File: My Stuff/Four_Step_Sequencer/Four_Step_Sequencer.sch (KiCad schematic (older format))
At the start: 46 parts, among them J1 CK_In, J10 1w, J11 2w, J12 3w, J13 4w, J2 CV_Out, J3 +12V_Conn, J4 GND_Conn, J5 -12V_Conn, J6 1a, J7 2a, J8 3a, J9 4a, U1 TL074, U2 4017

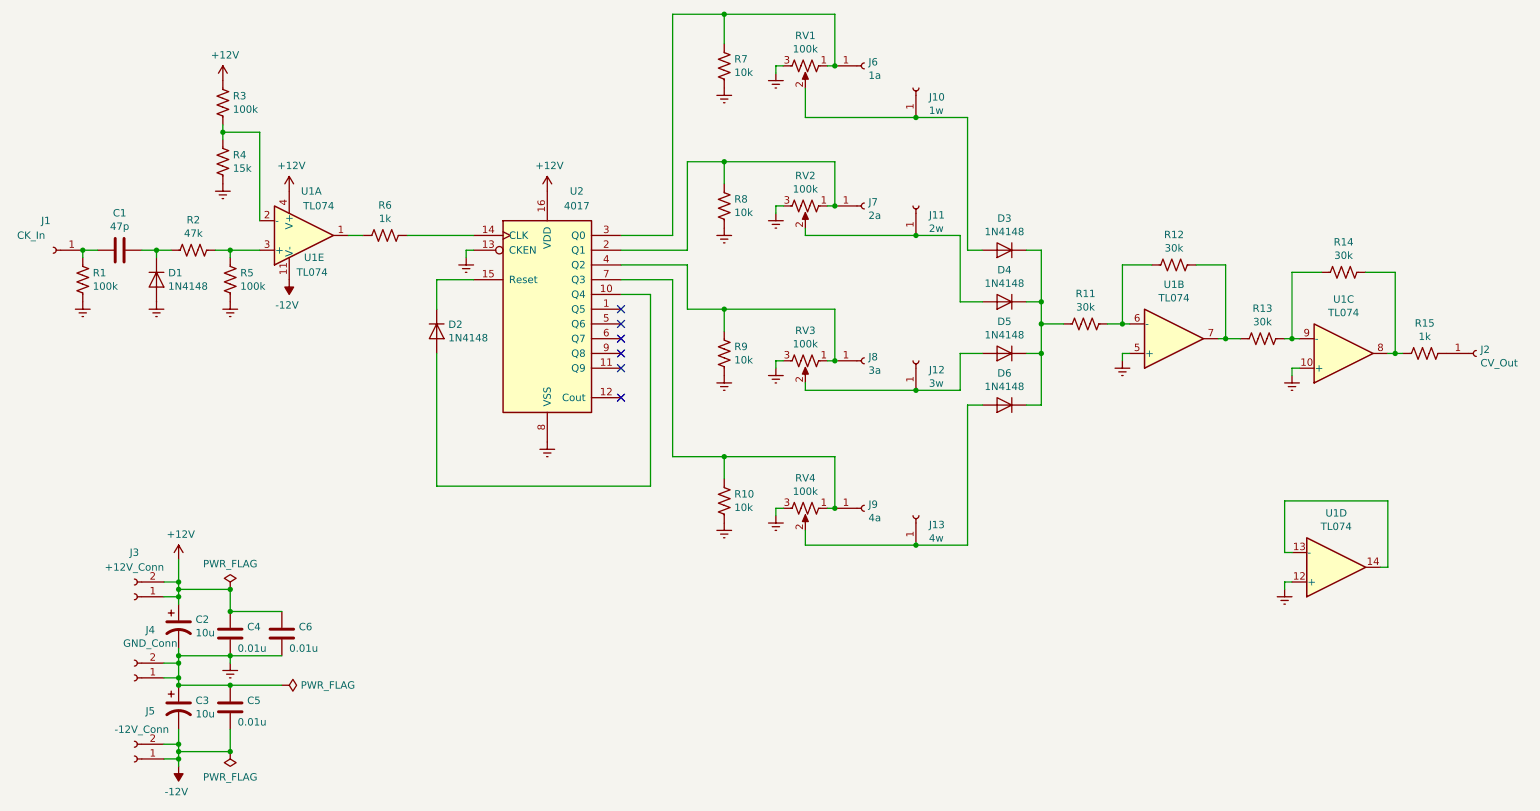
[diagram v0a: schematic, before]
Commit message: uwu
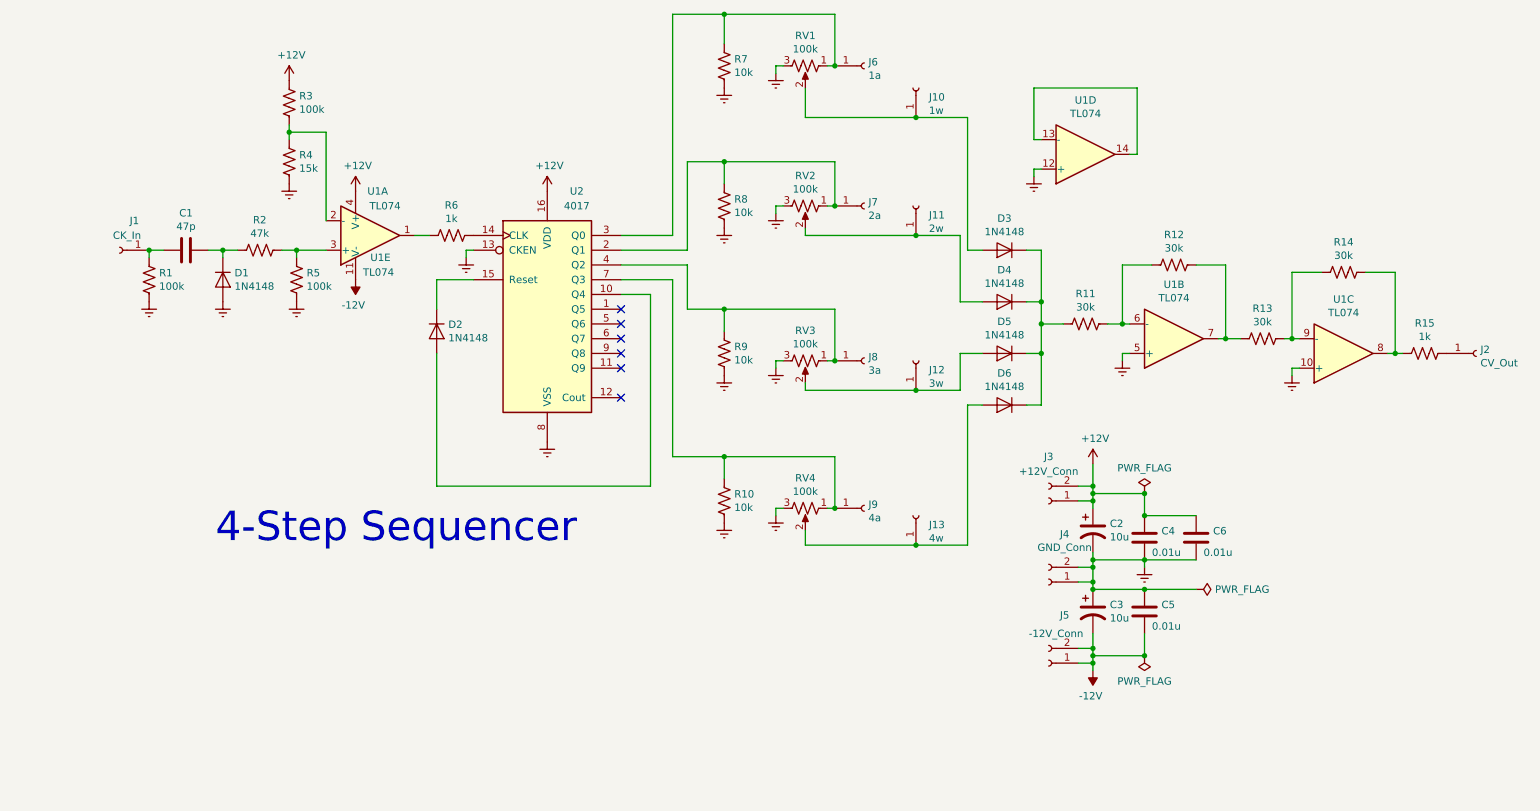
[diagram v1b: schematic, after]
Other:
- note added: "4-Step Sequencer\n"
- moved on the sheet: C1, C2, C3, C4, C5, C6, D1, J1, J3, J4, J5, R1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
